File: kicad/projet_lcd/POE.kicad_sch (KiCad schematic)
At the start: 83 parts, among them Q1 FOD817A3SD

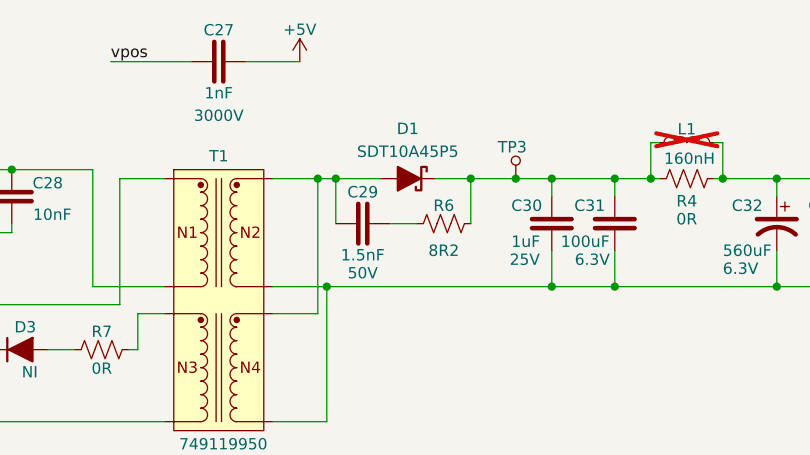
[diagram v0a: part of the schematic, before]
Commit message: schematiks seems okayish
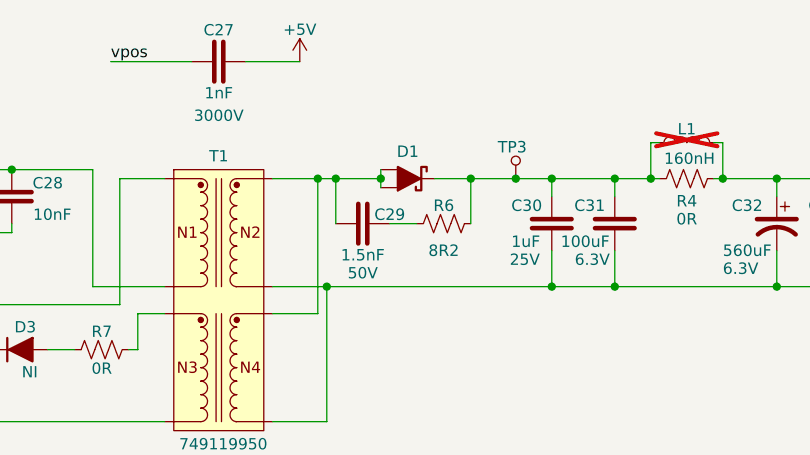
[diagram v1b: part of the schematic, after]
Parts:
- removed D1: SDT10A45P5, symbol Generics:D_Schottky
- added D1: ~, Diodes:SDT10A45P5, symbol Diodes:SDT10A45P5
- U3: footprint Voltage_Regulators:TL431 -> Voltage_regulators:TL431
- U4, U9: footprint Voltage_Regulators:AMS1117-3.3 -> Voltage_regulators:AMS1117-3.3
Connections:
- net GND: now also U3.A, U4.1 (Gnd), U9.1 (Gnd); no longer U3.2 (A), U4.Gnd, U9.Gnd
- net VSS: now also Q1.3 (E); no longer Q1.E
- net at C52.2, U3.K: now also Q1.2 (K); no longer Q1.K
- net at R13.1: now also Q1.1 (A); no longer Q1.A
- net at R12.1, R17.2 (1), TP10.1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: now also Q1.4 (C); no longer Q1.C
- net at C29.2, T1.7, T1.8: now also D1.A1 (A), D1.A2 (A)
- net at C30.2, C31.2, L1.1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: now also D1.K
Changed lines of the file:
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@@
 	)
 	(junction
+		(at 202 52)
+		(diameter 0)
+		(color 0 0 0 0)
+	)
+	(junction
 		(at 52 150)
 		(diameter 0)
@@
 	(wire
 		(pts
+			(xy 202 51) (xy 202 52)
+		)
+		(stroke
+			(width 0)
+			(type default)
+		)
+	)
+	(wire
+		(pts
 			(xy 166 104) (xy 166 106)
 		)
@@
 	(wire
 		(pts
+			(xy 202 52) (xy 202 53)
+		)
+		(stroke
+			(width 0)
+			(type default)
+		)
+	)
+	(wire
+		(pts
 			(xy 196 64) (xy 221 64)
 		)
@@
 			)
 		)
-		(pin "E"
+		(pin "2"
 		)
-		(pin "C"
+		(pin "1"
 		)
-		(pin "A"
+		(pin "4"
 		)
-		(pin "K"
+		(pin "3"
 		)
 		(instances
@@
 		(dnp no)
 		(property "Reference" "C29"
-			(at 200 53.5 0)
+			(at 203 56 0)
 			(effects
 				(font
@@
 	)
 	(symbol
-		(lib_id "Generics:D_Schottky")
-		(at 202 52 0)
-		(unit 1)
-		(exclude_from_sim no)
-		(in_bom yes)
-		(on_board yes)
-		(dnp no)
-		(property "Reference" "D1"
-			(at 205 46.46 0)
-			(effects
-				(font
-					(size 1.27 1.27)
-				)
-			)
-		)
-		(property "Value" "SDT10A45P5"
-			(at 205 49 0)
-			(effects
-				(font
-					(size 1.27 1.27)
-					(color 255 153 0 1)
-				)
-			)
-		)
-		(property "Footprint" ""
-			(at 205 52 0)
-			(effects
-				(font
-					(size 1.25 1.25)
-				)
-				(hide yes)
-			)
-		)
-		(property "Datasheet" ""
-			(at 202 59.4 0)
-			(effects
-				(font
-					(size 1.25 1.25)
-				)
-				(hide yes)
-			)
-		)
-		(property "Description" "Schottky diode"
-			(at 205 57 0)
-			(effects
-				(font
-					(size 1.25 1.25)
-				)
-				(hide yes)
-			)
-		)
-		(property "Part#" "NI"
-			(at 205.4785 47.67 0)
-			(effects
-				(font
-					(size 1.25 1.25)
-				)
-				(hide yes)
-			)
-		)
-		(property "Comments" ""
-			(at 205 52 0)
-			(effects
-				(font
-					(size 1.25 1.25)
-				)
-				(hide yes)
-			)
-		)
-		(property "LCSC Part #" "C5746878"
-			(at 202 52 0)
-			(effects
-				(font
-					(size 1.27 1.27)
-				)
-				(hide yes)
-			)
-		)
-		(pin "K"
-		)
-		(pin "A"
-		)
-		(instances
-			(project ""
-				(path "/b3ce22de-813e-4a84-80c2-bec39c904000/4cd1692b-280a-46ef-a0ce-bb76541e4c5a"
-					(reference "D1")
-					(unit 1)
-				)
-			)
-		)
-	)
-	(symbol
 		(lib_id "Generics:R")
 		(at 168 71 0)
@@
 	)
 	(symbol
+		(lib_id "Diodes:SDT10A45P5")
+		(at 205 52 0)
+		(unit 1)
+		(exclude_from_sim no)
+		(in_bom yes)
+		(on_board yes)
+		(dnp no)
+		(property "Reference" "D1"
+			(at 205 49 0)
+			(effects
+				(font
+					(size 1.27 1.27)
+				)
+			)
+		)
+		(property "Value" "~"
+			(at 205.5 48.26 0)
+			(effects
+				(font
+					(size 1.27 1.27)
+				)
+				(hide yes)
+			)
+		)
+		(property "Footprint" "Diodes:SDT10A45P5"
+			(at 205 61 0)
+			(effects
+				(font
+					(size 1.27 1.27)
+				)
+				(hide yes)
+			)
+		)
+		(property "Datasheet" ""
+			(at 205 52 0)
+			(effects
+				(font
+					(size 1.27 1.27)
+				)
+				(hide yes)
+			)
+		)
+		(property "Description" "Schottky Barrier Rectifier 10A"
+			(at 205 57 0)
+			(effects
+				(font
+					(size 1.27 1.27)
+				)
+				(hide yes)
+			)
+		)
+		(property "LCSC Part#" "C5746878"
+			(at 205 59 0)
+			(effects
+				(font
+					(size 1.27 1.27)
+				)
+				(hide yes)
+			)
+		)
+		(pin "A2"
+		)
+		(pin "A1"
+		)
+		(pin "K"
+		)
+		(instances
+			(project ""
+				(path "/b3ce22de-813e-4a84-80c2-bec39c904000/4cd1692b-280a-46ef-a0ce-bb76541e4c5a"
+					(reference "D1")
+					(unit 1)
+				)
+			)
+		)
+	)
+	(symbol
 		(lib_id "Generics:D")
 		(at 35 82 90)
@@
 			)
 		)
-		(property "Footprint" "Voltage_Regulators:AMS1117-3.3"
+		(property "Footprint" "Voltage_regulators:AMS1117-3.3"
 			(at 70 175 0)
 			(effects
@@
 		(pin "4"
 		)
-		(pin "Gnd"
+		(pin "1"
 		)
 		(pin "2"
@@
 			)
 		)
-		(property "Footprint" "Voltage_Regulators:TL431"
+		(property "Footprint" "Voltage_regulators:TL431"
 			(at 187 123 0)
 			(effects
@@
 		(pin "K"
 		)
-		(pin "2"
+		(pin "A"
 		)
 		(pin "Ref"
@@
 			)
 		)
-		(property "Footprint" "Voltage_Regulators:AMS1117-3.3"
+		(property "Footprint" "Voltage_regulators:AMS1117-3.3"
 			(at 70 150 0)
 			(effects
@@
 		(pin "4"
 		)
-		(pin "Gnd"
+		(pin "1"
 		)
 		(pin "2"
